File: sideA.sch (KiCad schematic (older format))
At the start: 18 parts, among them J1 USB_2, P1 CONN_2, Q1 NPN, Q2 NPN, Q3 NPN, SW1 SW_PUSH, SW2 SW_PUSH, SW3 SW_PUSH

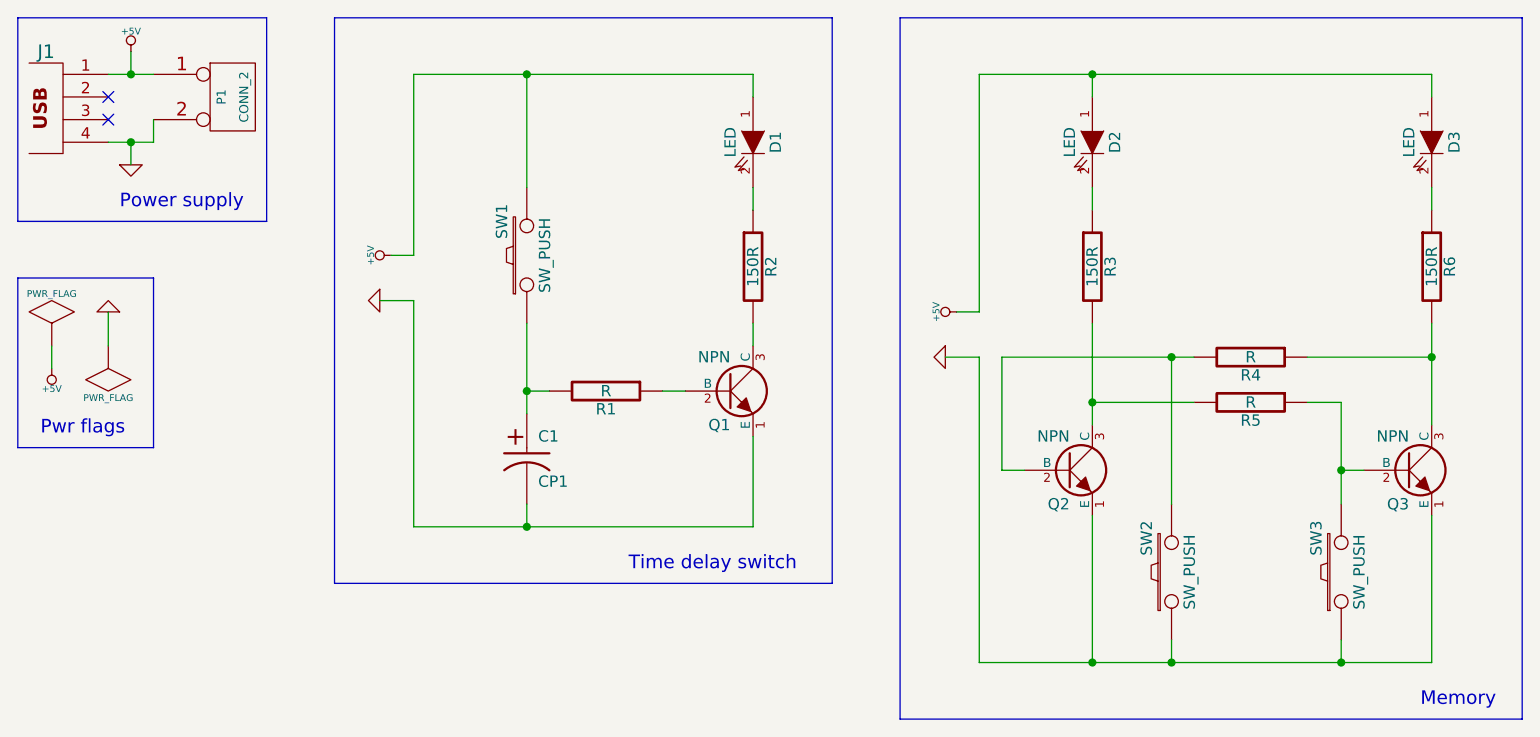
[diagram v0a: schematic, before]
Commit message: All components spitted on the board.
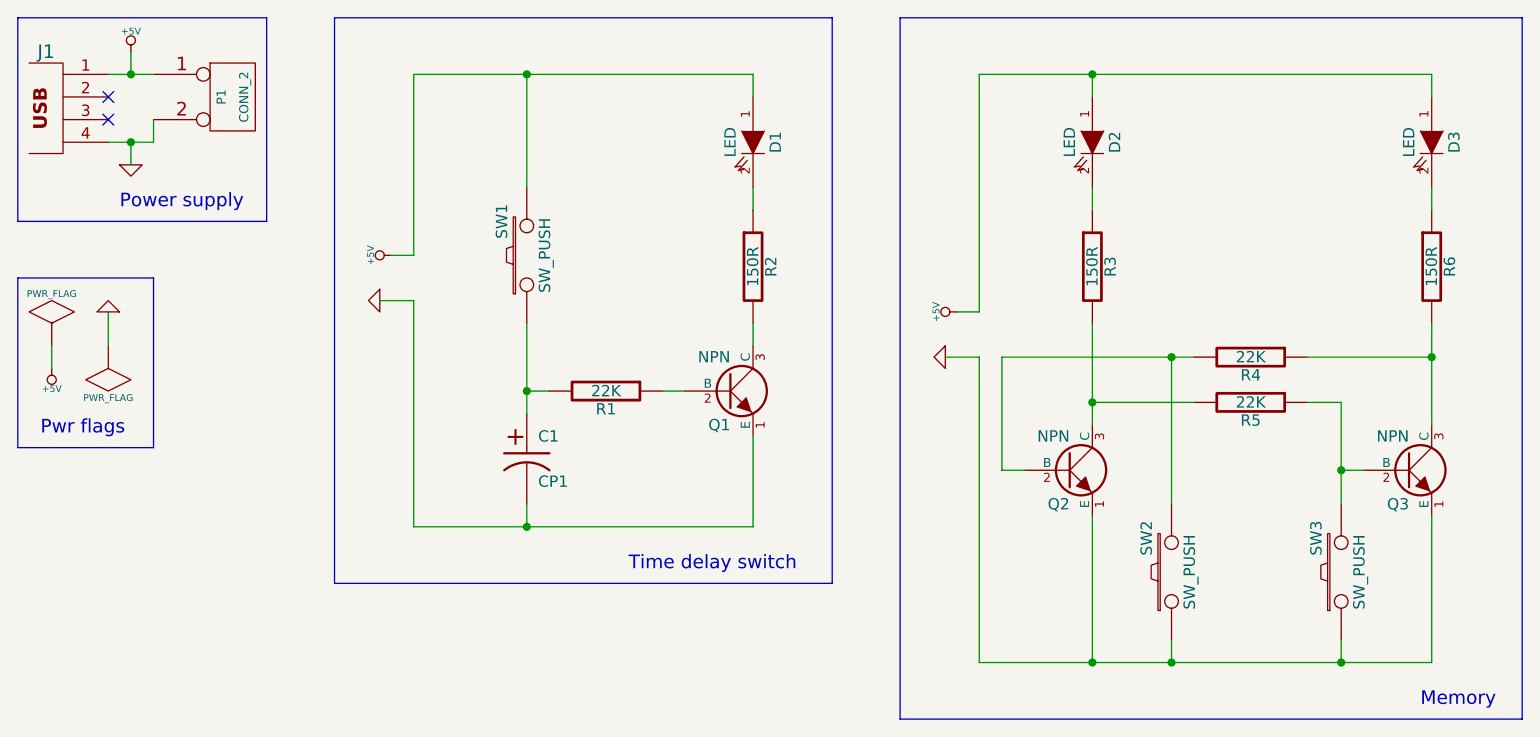
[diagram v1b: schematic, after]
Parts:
- R1, R4, R5: value R -> 22K
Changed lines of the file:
@@
-EESchema Schematic File Version 2  date Tue 26 Feb 2013 22:56:48 CET
+EESchema Schematic File Version 2  date Wed 27 Feb 2013 15:39:57 CET
 LIBS:power
 LIBS:device
@@
 Sheet 1 1
 Title "SMT4dummies - sideA"
-Date "26 feb 2013"
+Date "27 feb 2013"
 Rev ""
 Comp "d-Squared Robotics"
@@
 P 6550 2600
 F 0 "R4" V 6630 2600 50  0000 C CNN
-F 1 "R" V 6550 2600 50  0000 C CNN
+F 1 "22K" V 6550 2600 50  0000 C CNN
 	1    6550 2600
 	0    1    1    0
@@
 P 6550 2800
 F 0 "R5" V 6630 2800 50  0000 C CNN
-F 1 "R" V 6550 2800 50  0000 C CNN
+F 1 "22K" V 6550 2800 50  0000 C CNN
 	1    6550 2800
 	0    1    1    0
@@
 P 3700 2750
 F 0 "R1" V 3780 2750 50  0000 C CNN
-F 1 "R" V 3700 2750 50  0000 C CNN
+F 1 "22K" V 3700 2750 50  0000 C CNN
 	1    3700 2750
 	0    1    1    0
